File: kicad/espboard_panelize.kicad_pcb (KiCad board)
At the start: 2 copper layers, 66 x 40.6 mm, 17 parts, among them J1 USB_OTG, P1 ftdi, P2 CONN_PWR, P3 CONN_IO, P4 usb_connector, U1 ESP-01v090, U2 LM1117-3.3

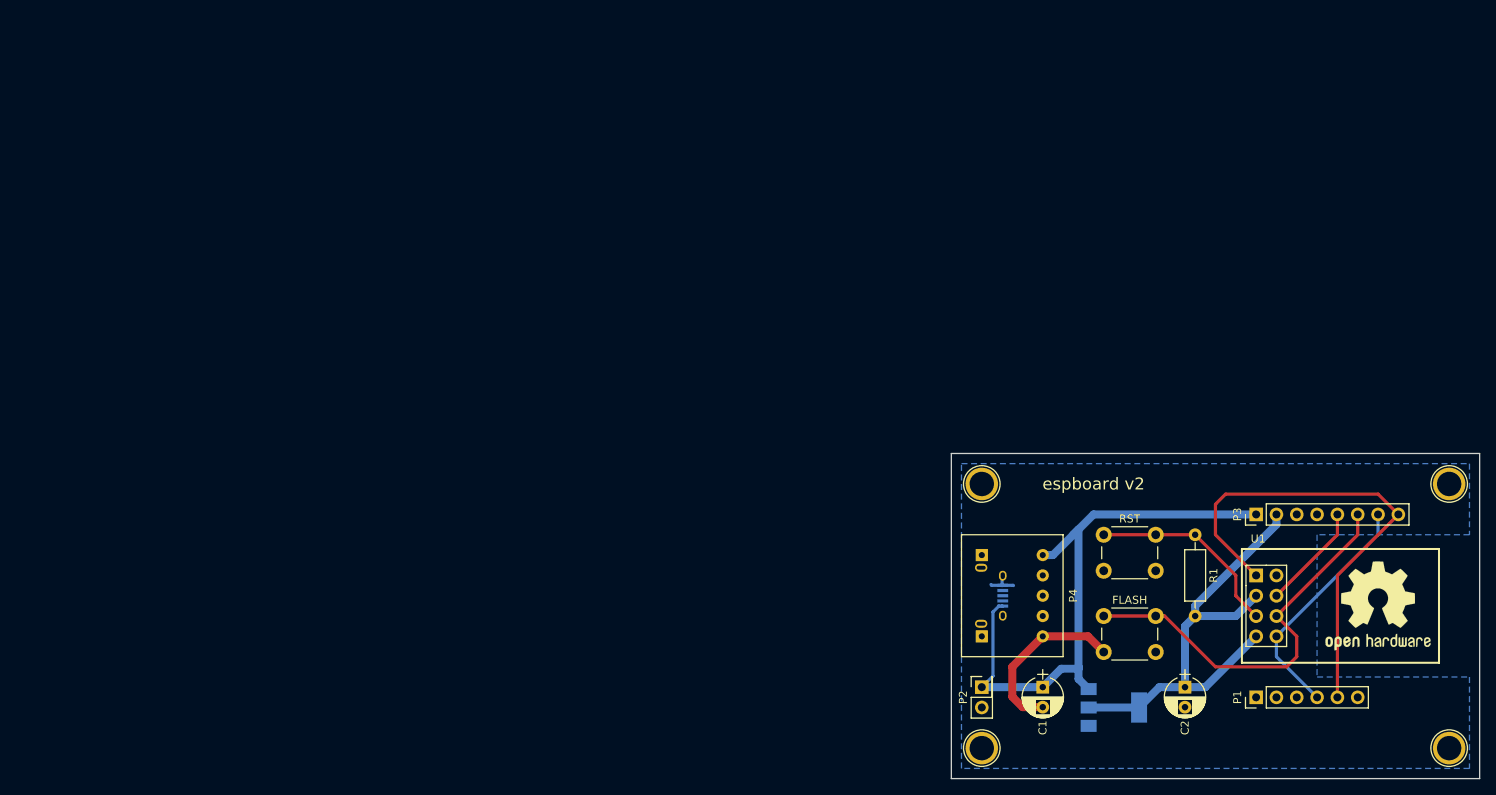
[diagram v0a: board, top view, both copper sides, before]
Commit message: v2
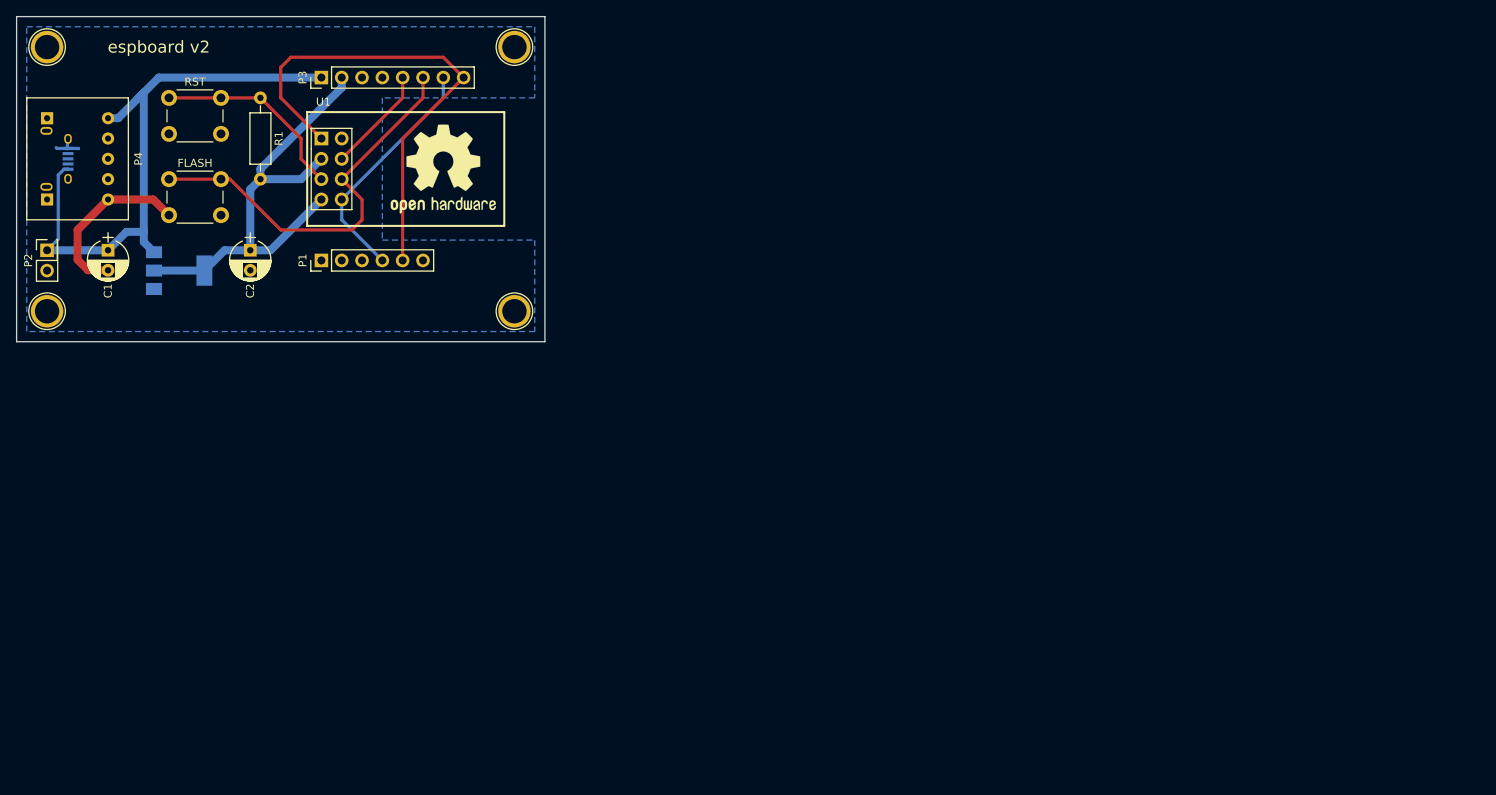
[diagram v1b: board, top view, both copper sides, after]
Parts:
- moved REF** 129.0 mm to (92.7, 27.9)
- moved REF** 129.0 mm to (92.7, 61.0)
- moved C1 129.0 mm to (41.9, 53.3)
- moved C2 129.0 mm to (59.7, 53.3)
- moved FLASH 129.0 mm to (49.5, 44.5)
- moved J1 129.0 mm to (35.6, 41.9)
- moved P1 129.0 mm to (68.6, 54.6)
- moved P2 129.0 mm to (34.3, 53.3)
- moved P3 129.0 mm to (68.6, 31.8)
- moved P4 129.0 mm to (41.9, 41.9)
- moved R1 129.0 mm to (61.0, 34.3)
- moved REF** 129.0 mm to (34.3, 61.0)
- moved REF** 129.0 mm to (34.3, 27.9)
- moved REF*** 129.0 mm to (83.8, 43.2)
- moved RST 129.0 mm to (49.5, 34.3)
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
